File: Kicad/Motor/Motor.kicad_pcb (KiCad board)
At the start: 2 copper layers, 7 parts, among them J1 12V, J2 PWM, J3 Motor 12V, J4 Motor Ground, J5 Ground, Q1 TIP120

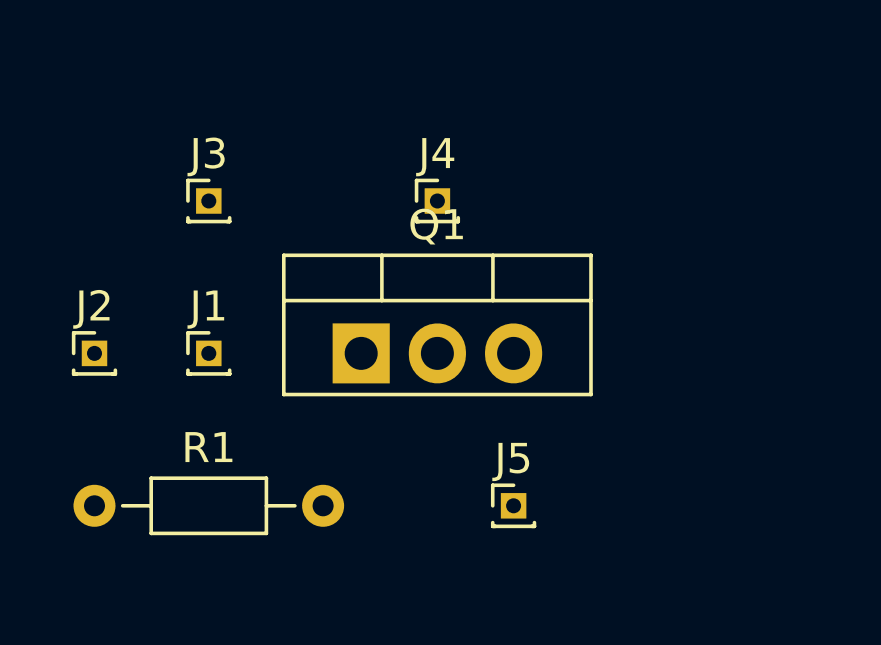
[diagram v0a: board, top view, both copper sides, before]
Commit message: Update
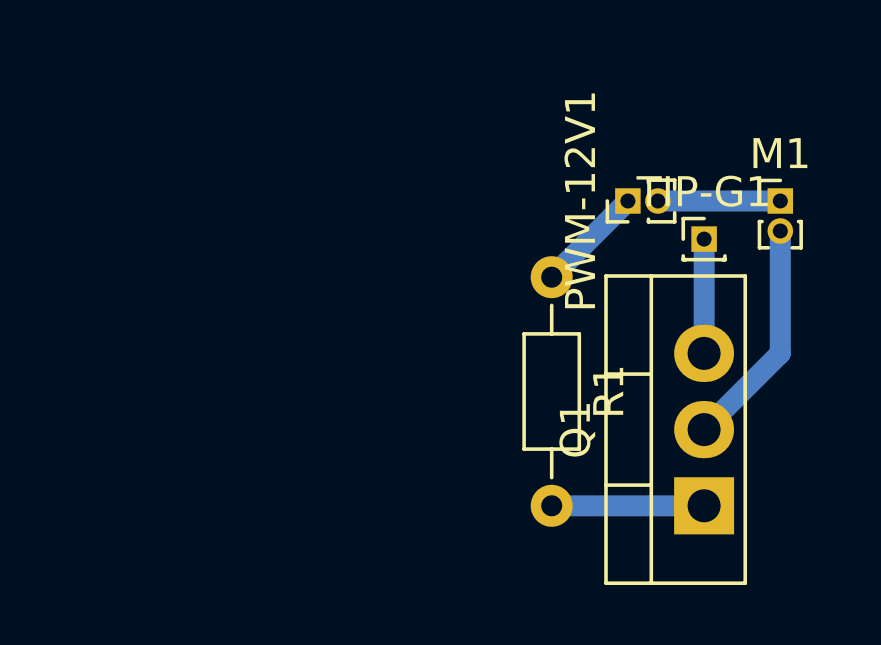
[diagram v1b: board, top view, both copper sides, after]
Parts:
- removed J1: 12V, Connector_PinHeader_1.00mm:PinHeader_1x01_P1.00mm_Vertical
- removed J2: PWM, Connector_PinHeader_1.00mm:PinHeader_1x01_P1.00mm_Vertical
- removed J3: Motor 12V, Connector_PinHeader_1.00mm:PinHeader_1x01_P1.00mm_Vertical
- removed J4: Motor Ground, Connector_PinHeader_1.00mm:PinHeader_1x01_P1.00mm_Vertical
- removed J5: Ground, Connector_PinHeader_1.00mm:PinHeader_1x01_P1.00mm_Vertical
- added M1: M 12V og M Gorund, Connector_PinHeader_1.00mm:PinHeader_1x02_P1.00mm_Vertical, F.Cu at (153.7, 91.4)
- added PWM-12V1: PWM og 12V, Connector_PinHeader_1.00mm:PinHeader_1x02_P1.00mm_Vertical, F.Cu at (148.6, 91.4)
- added TIP-G1: Ground, Connector_PinHeader_1.00mm:PinHeader_1x01_P1.00mm_Vertical, F.Cu at (151.1, 92.7)
- moved R1 17.0 mm to (146.1, 94.0), turned to -90 degrees
- moved Q1 12.5 mm to (151.1, 101.6), turned to 90 degrees
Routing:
- net Net-(Q1-Pad2): track 0.00 -> 7.67 mm
- net Net-(Q1-Pad1): track 0.00 -> 5.08 mm
- net Net-(PWM-12V1-Pad2): track 0.00 -> 4.08 mm
- net Net-(TIP-G1-Pad1): track 0.00 -> 3.81 mm
- net Net-(R1-Pad1): track 0.00 -> 3.59 mm
